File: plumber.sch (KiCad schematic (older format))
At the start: 99 parts, among them IC1 MP2451DT-LF-Z, J1 Conn_01x03, J2 Conn_01x03, J3 Conn_01x03, J4 Conn_01x03, J5 Conn_01x02, J6 Conn_01x02, J7 Conn_01x02, J8 Conn_01x02, J9 Conn_01x02, K1 ADW1103HLW, K2 ADW1103HLW, K3 ADW1103HLW, K4 ADW1103HLW, Q1 Si2319CDS, Q10 2N7002, Q11 Si2319CDS, Q12 2N7002, Q13 Si2319CDS, Q14 2N7002, Q15 Si2319CDS, Q16 2N7002, Q2 2N7002, Q3 Si2319CDS, Q4 2N7002, Q5 Si2319CDS, Q6 2N7002, Q7 Si2319CDS, Q8 2N7002, Q9 Si2319CDS, U1 ESP-12F

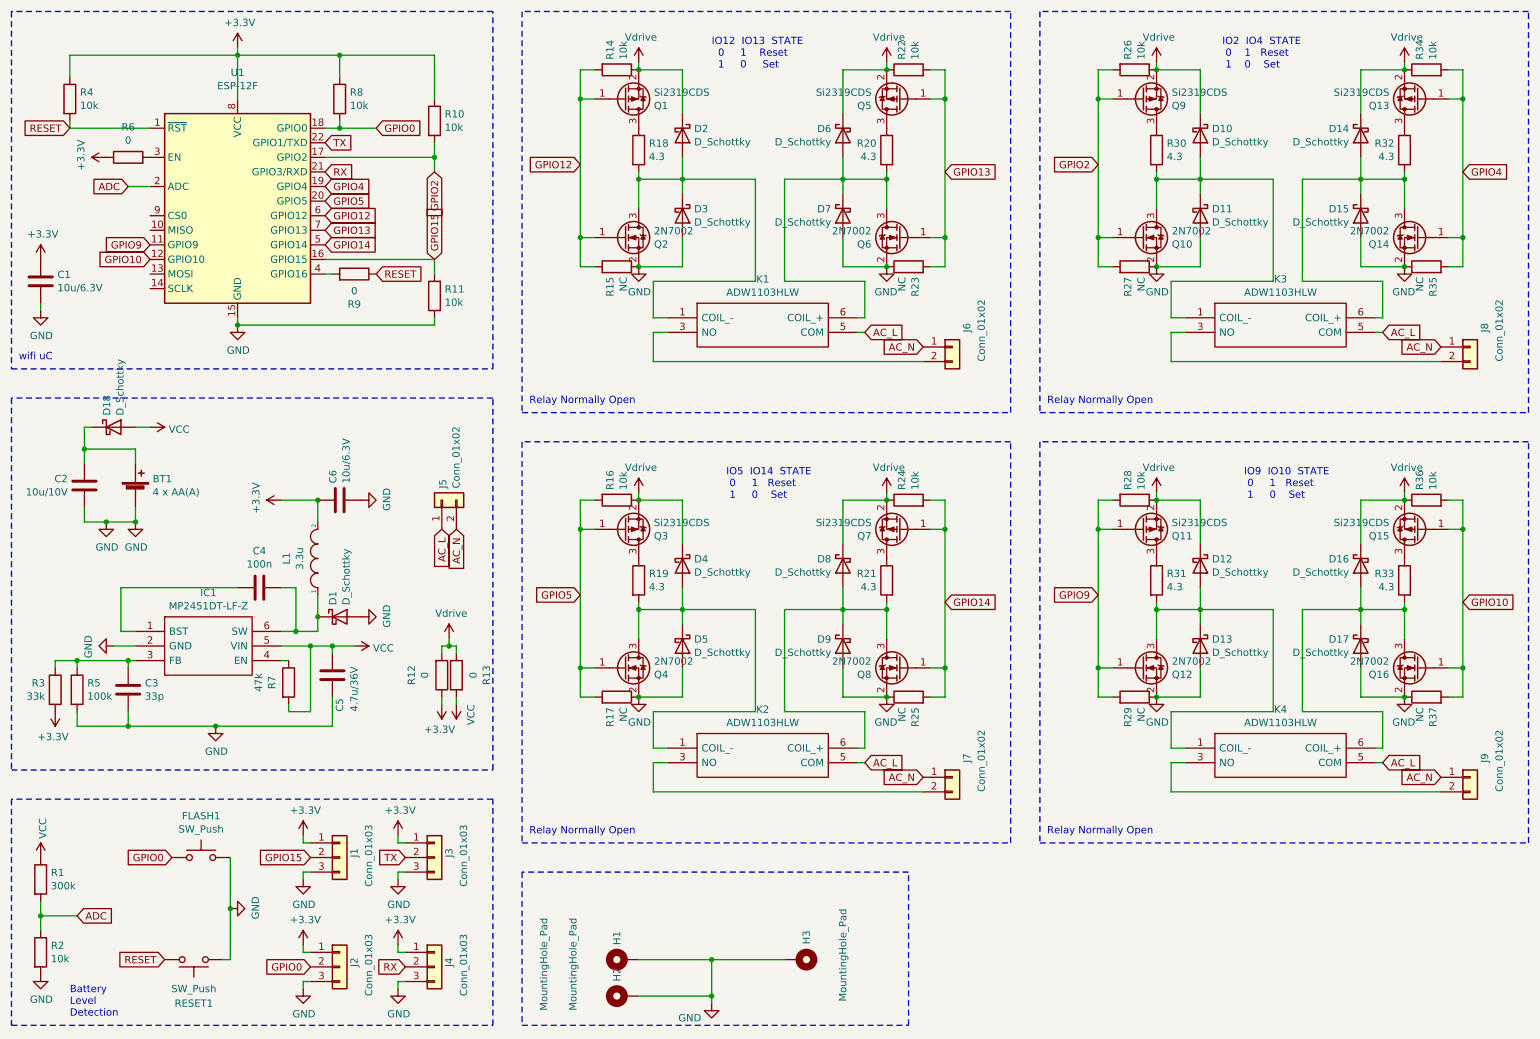
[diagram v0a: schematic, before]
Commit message: hardware v1
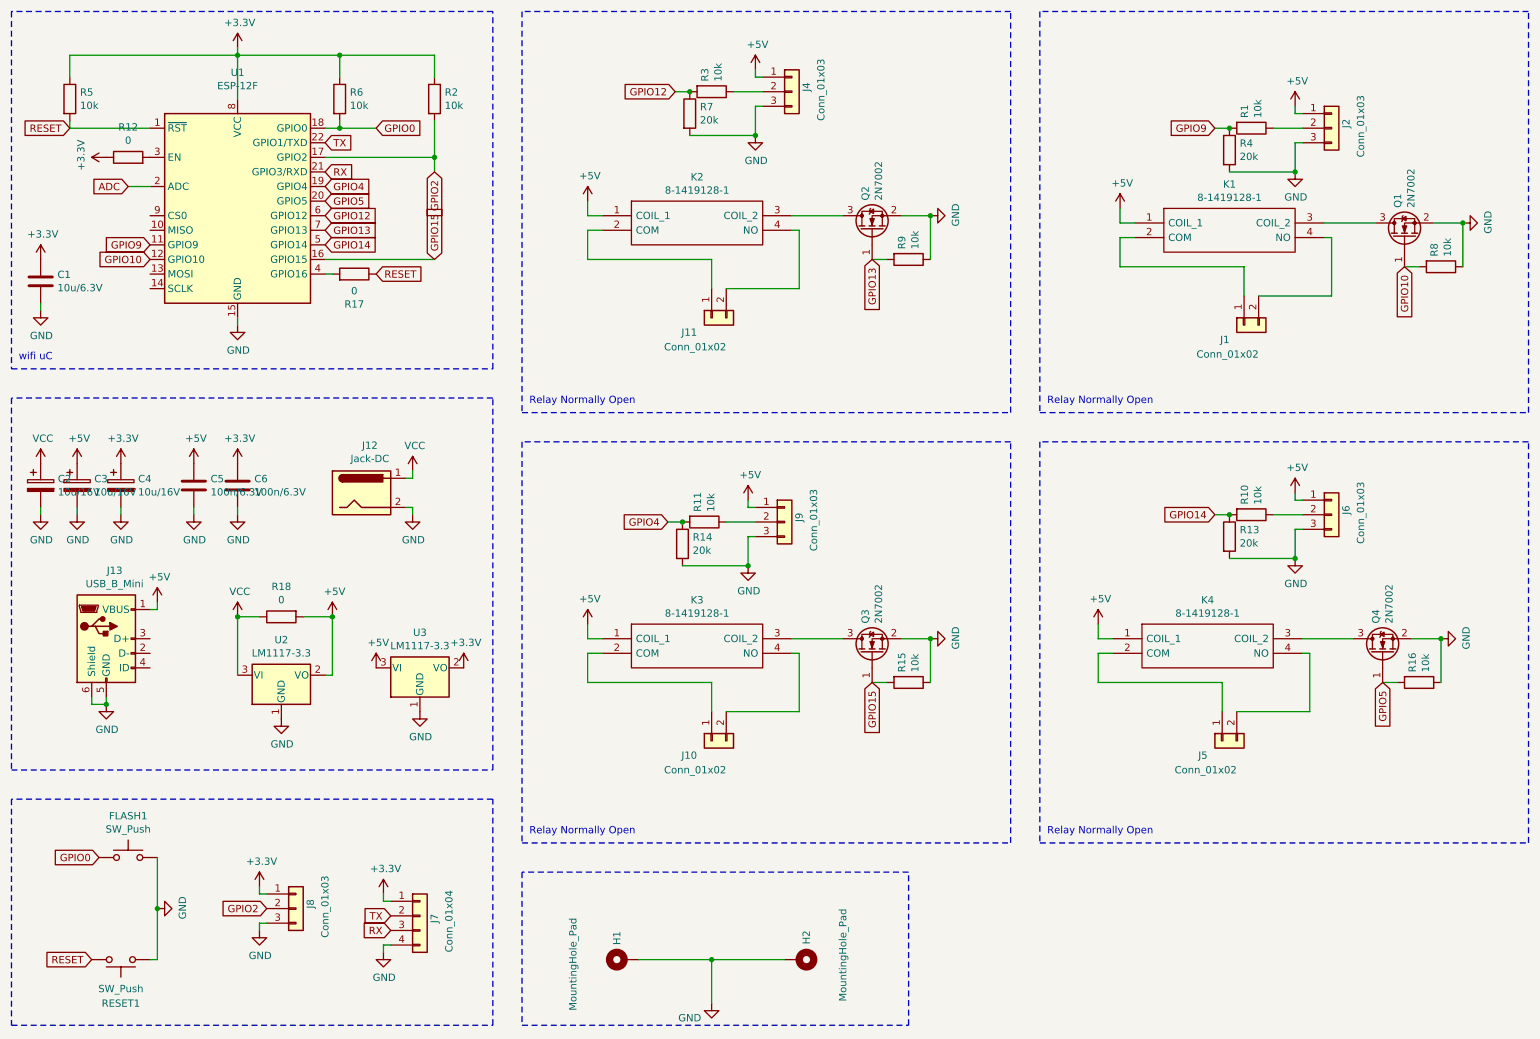
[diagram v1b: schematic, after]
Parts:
- removed BT1: 4 x AA(A), Connector_PinHeader_2.54mm:PinHeader_1x02_P2.54mm_Vertical, symbol Device:Battery_Cell
- removed C2: 10u/10V, Capacitor_SMD:C_0603_1608Metric, symbol Device:C
- removed C3: 33p, Capacitor_SMD:C_0402_1005Metric, symbol Device:C
- removed C4: 100n, Capacitor_SMD:C_0402_1005Metric, symbol Device:C
- removed D1, D10, D11, D12, D13, D14, D15, D16, D17, D18, D2, D3, D4, D5, D6, D7, D8, D9: D_Schottky, Diode_SMD:D_SOD-123, symbol Device:D_Schottky
- removed H2: MountingHole_Pad, MountingHole:MountingHole_3.7mm_Pad, symbol Mechanical:MountingHole_Pad
- removed IC1: MP2451DT-LF-Z, SamacSys_Parts:SOT95P280X145-6N, symbol SamacSys_Parts:MP2451DT-LF-Z
- removed J1, J3: Conn_01x03, Connector_Harwin:Harwin_M20-89003xx_1x03_P2.54mm_Horizontal, symbol Connector_Generic:Conn_01x03
- removed J7, J8, J9: Conn_01x02, TerminalBlock_Phoenix:TerminalBlock_Phoenix_MKDS-1,5-2_1x02_P5.00mm_Horizontal, symbol Connector_Generic:Conn_01x02
- removed K1, K2, K3, K4: ADW1103HLW, SamacSys_Parts:ADW1103HLW, symbol SamacSys_Parts:ADW1103HLW
- removed L1: 3.3u, Inductor_SMD:L_Bourns-SRN4018, symbol pspice:INDUCTOR
- removed Q1, Q11, Q13, Q15, Q3, Q5, Q7, Q9: Si2319CDS, Package_TO_SOT_SMD:SOT-23, symbol Transistor_FET:Si2319CDS
- removed Q10, Q12, Q14, Q16, Q6, Q8: 2N7002, Package_TO_SOT_SMD:SOT-23, symbol Transistor_FET:2N7002
- removed R12: 0, Resistor_SMD:R_0402_1005Metric, symbol Device:R
- removed R17, R23, R25, R27, R29, R35, R37: NC, Resistor_SMD:R_0402_1005Metric, symbol Device:R
- removed R19, R20, R21, R30, R31, R32, R33: 4.3, Resistor_SMD:R_0603_1608Metric, symbol Device:R
- removed R22, R24, R26, R28, R34, R36: 10k, Resistor_SMD:R_0402_1005Metric, symbol Device:R
- removed R5: 100k, Resistor_SMD:R_0402_1005Metric, symbol Device:R
- added C2, C3, C4: 10u/16V, Capacitor_THT:CP_Radial_D8.0mm_P3.50mm, symbol Device:CP
- added J10, J11: Conn_01x02, TerminalBlock_Phoenix:TerminalBlock_Phoenix_MKDS-1,5-2_1x02_P5.00mm_Horizontal, symbol Connector_Generic:Conn_01x02
- added J12: Jack-DC, Connector_BarrelJack:BarrelJack_Horizontal, symbol Connector:Jack-DC
- added J13: USB_B_Mini, Connector_USB:USB_Micro-B_Molex-105017-0001, symbol Connector:USB_B_Mini
- added J2, J6, J9: Conn_01x03, Connector_PinSocket_2.54mm:PinSocket_1x03_P2.54mm_Vertical, symbol Connector_Generic:Conn_01x03
- added J7: Conn_01x04, Connector_PinSocket_2.54mm:PinSocket_1x04_P2.54mm_Vertical, symbol Connector_Generic:Conn_01x04
- added K1, K2, K3, K4: 8-1419128-1, SamacSys_Parts:814191281, symbol SamacSys_Parts:8-1419128-1
- added Q1, Q3: 2N7002, Package_TO_SOT_SMD:SOT-23, symbol Transistor_FET:2N7002
- added R4: 20k, Resistor_SMD:R_0603_1608Metric_Pad0.98x0.95mm_HandSolder, symbol Device:R
- added R8, R9: 10k, Resistor_SMD:R_0603_1608Metric_Pad0.98x0.95mm_HandSolder, symbol Device:R
- added U2, U3: LM1117-3.3, Package_TO_SOT_SMD:SOT-223-3_TabPin2, symbol Regulator_Linear:LM1117-3.3
- C1: footprint Capacitor_SMD:C_0402_1005Metric -> Capacitor_SMD:C_0603_1608Metric_Pad1.08x0.95mm_HandSolder
- C5: value 4.7u/36V -> 100n/6.3V; footprint Capacitor_SMD:C_1206_3216Metric -> Capacitor_SMD:C_0603_1608Metric_Pad1.08x0.95mm_HandSolder
- C6: value 10u/6.3V -> 100n/6.3V; footprint Capacitor_SMD:C_0402_1005Metric -> Capacitor_SMD:C_0603_1608Metric_Pad1.08x0.95mm_HandSolder
- FLASH1, RESET1: footprint Button_Switch_SMD:SW_SPST_EVQP7A -> Button_Switch_SMD:SW_SPST_EVQPE1
- J4: footprint Connector_Harwin:Harwin_M20-89003xx_1x03_P2.54mm_Horizontal -> Connector_PinSocket_2.54mm:PinSocket_1x03_P2.54mm_Vertical
- J8: renamed from J2; footprint Connector_Harwin:Harwin_M20-89003xx_1x03_P2.54mm_Horizontal -> Connector_PinSocket_2.54mm:PinSocket_1x03_P2.54mm_Vertical
- R1: value 300k -> 10k; footprint Resistor_SMD:R_0402_1005Metric -> Resistor_SMD:R_0603_1608Metric_Pad0.98x0.95mm_HandSolder
- R10, R11, R16, R2: footprint Resistor_SMD:R_0402_1005Metric -> Resistor_SMD:R_0603_1608Metric_Pad0.98x0.95mm_HandSolder
- R12: renamed from R6; footprint Resistor_SMD:R_0402_1005Metric -> Resistor_SMD:R_0603_1608Metric_Pad0.98x0.95mm_HandSolder
- R13: value 0 -> 20k; footprint Resistor_SMD:R_0402_1005Metric -> Resistor_SMD:R_0603_1608Metric_Pad0.98x0.95mm_HandSolder
- R14: value 10k -> 20k; footprint Resistor_SMD:R_0402_1005Metric -> Resistor_SMD:R_0603_1608Metric_Pad0.98x0.95mm_HandSolder
- R15: value NC -> 10k; footprint Resistor_SMD:R_0402_1005Metric -> Resistor_SMD:R_0603_1608Metric_Pad0.98x0.95mm_HandSolder
- R17: renamed from R9; footprint Resistor_SMD:R_0402_1005Metric -> Resistor_SMD:R_0603_1608Metric_Pad0.98x0.95mm_HandSolder
- R18: value 4.3 -> 0; footprint Resistor_SMD:R_0603_1608Metric -> Resistor_SMD:R_0603_1608Metric_Pad0.98x0.95mm_HandSolder
- R3: value 33k -> 10k; footprint Resistor_SMD:R_0402_1005Metric -> Resistor_SMD:R_0603_1608Metric_Pad0.98x0.95mm_HandSolder
- R5: renamed from R4; footprint Resistor_SMD:R_0402_1005Metric -> Resistor_SMD:R_0603_1608Metric_Pad0.98x0.95mm_HandSolder
- R6: renamed from R8; footprint Resistor_SMD:R_0402_1005Metric -> Resistor_SMD:R_0603_1608Metric_Pad0.98x0.95mm_HandSolder
- R7: value 47k -> 20k; footprint Resistor_SMD:R_0402_1005Metric -> Resistor_SMD:R_0603_1608Metric_Pad0.98x0.95mm_HandSolder
- renumbered H3 to H2, J6 to J1
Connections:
- net +3V3: now also R2.1, C4.1, J7.1 (Pin_1), U3.2 (VO); no longer J4.1 (Pin_1), R10.1, R3.2
- net ADC: no longer R1.2, R2.1
- net GND: now also R13.2, R14.2, R16.1, R7.2, C2.2, C3.2, C4.2, J12.2, J13.5 (GND), J13.6 (Shield), J2.3 (Pin_3), J6.3 (Pin_3), J7.4 (Pin_4), J9.3 (Pin_3), Q1.2 (S), Q3.2 (S), R4.2, R8.1, R9.1, U2.1 (GND), U3.1 (GND); no longer R11.1, R2.2
- net GPIO0: no longer J8.2 (Pin_2)
- net GPIO10: now also Q1.1 (G), R8.2
- net GPIO12: now also R3.2, R7.1; no longer Q2.1 (G), R14.2, R15.2
- net GPIO13: now also Q2.1 (G), R9.2
- net GPIO14: now also R10.2, R13.1
- net GPIO15: now also R15.2, Q3.1 (G); no longer R11.2
- net GPIO2: now also J8.2 (Pin_2), R2.2; no longer R10.2
- net GPIO4: now also R11.2, R14.1
- net GPIO9: now also R1.2, R4.1
- net RX: now also J7.3 (Pin_3); no longer J4.2 (Pin_2)
- net TX: now also J7.2 (Pin_2)
- net VCC: now also R18.1, C2.1, J12.1, U2.3 (VI); no longer C5.1, R1.1, R13.2, R7.2
- net at Q4.3 (D): now also K4.3 (COIL_2)
- net at R3.1: now also J4.2 (Pin_2)
- net at Q2.3 (D): now also K2.3 (COIL_2); no longer R18.2
- net at J1.2 (Pin_2): now also K1.4 (NO)
- net AC_L: no longer names the net of J5.1 (Pin_1)
- net AC_L: now also K4.2 (COM)
- net AC_N: no longer names the net of J1.1 (Pin_1)
- net AC_N: now also K1.2 (COM); no longer J5.2 (Pin_2)
- removed net Vdrive: R13.1, R14.1, R16.1
- new net: J11.1 (Pin_1), K2.2 (COM)
- new net: J11.2 (Pin_2), K2.4 (NO)
- new net: K1.3 (COIL_2), Q1.3 (D)
- new net: J5.2 (Pin_2), K4.4 (NO)
- new net: J10.1 (Pin_1), K3.2 (COM)
- new net: K3.3 (COIL_2), Q3.3 (D)
- new net: J10.2 (Pin_2), K3.4 (NO)
- new net: J2.2 (Pin_2), R1.1
- new net: J6.2 (Pin_2), R10.1
- new net: J9.2 (Pin_2), R11.1
- new net +5V: C3.1, C5.1, J13.1 (VBUS), J2.1 (Pin_1), J4.1 (Pin_1), J6.1 (Pin_1), J9.1 (Pin_1), K1.1 (COIL_1), K2.1 (COIL_1), K3.1 (COIL_1), K4.1 (COIL_1), R18.2, U2.2 (VO), U3.3 (VI)
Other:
- note removed: "Battery\nLevel\nDetection"
- note removed: "IO12 IO13 STATE\n 0 1 Reset\n 1 0 Set"
- note removed: "IO2 IO4 STATE\n 0 1 Reset\n 1 0 Set"
- note removed: "IO5 IO14 STATE\n 0 1 Reset\n 1 0 Set"
- note removed: "IO9 IO10 STATE\n 0 1 Reset\n 1 0 Set"
- moved on the sheet: FLASH1, J1, J8, RESET1
